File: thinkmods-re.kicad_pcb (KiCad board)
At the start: 2 copper layers, 30.5 x 68.1 mm, 12 parts, among them J1 ExpressCard, J2 Bus_M.2_Socket_M, J3 Micro_SD_Card, U1 GL823K-HCY04

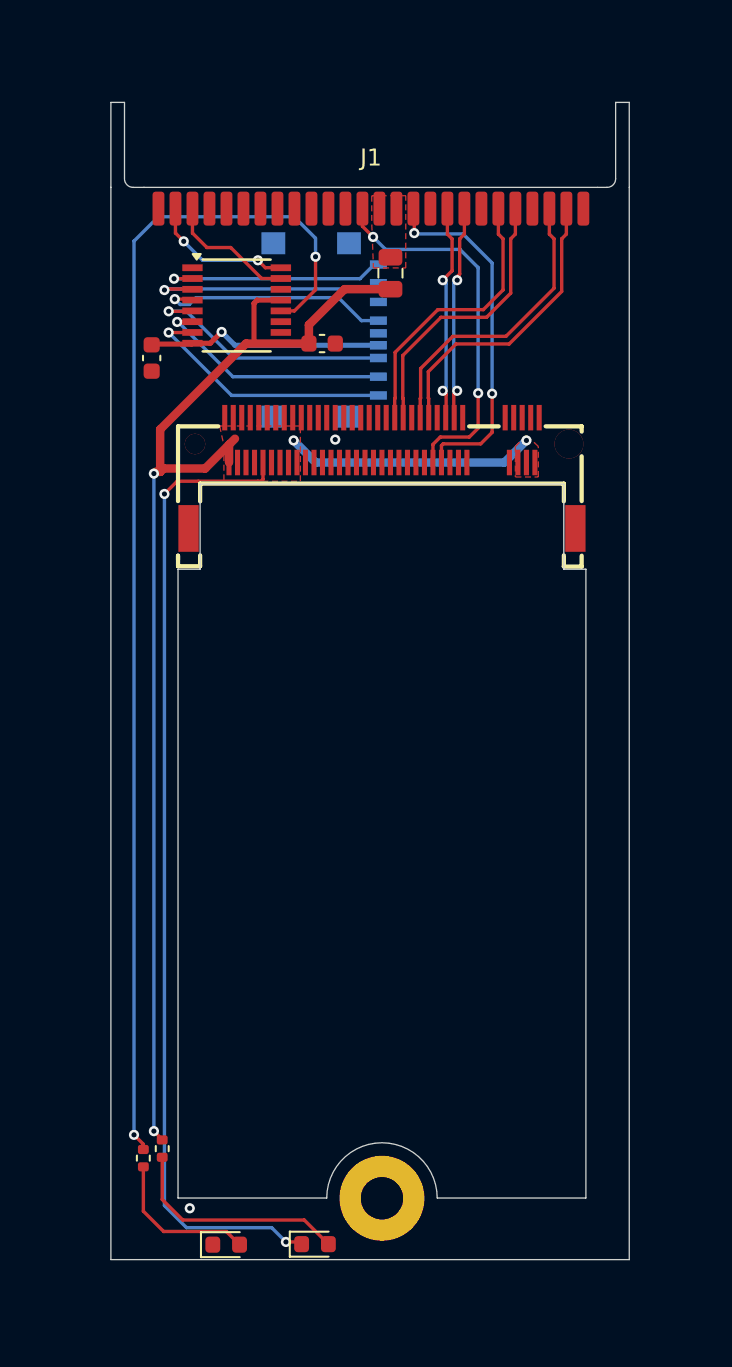
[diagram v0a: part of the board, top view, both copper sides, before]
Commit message: Add files via upload
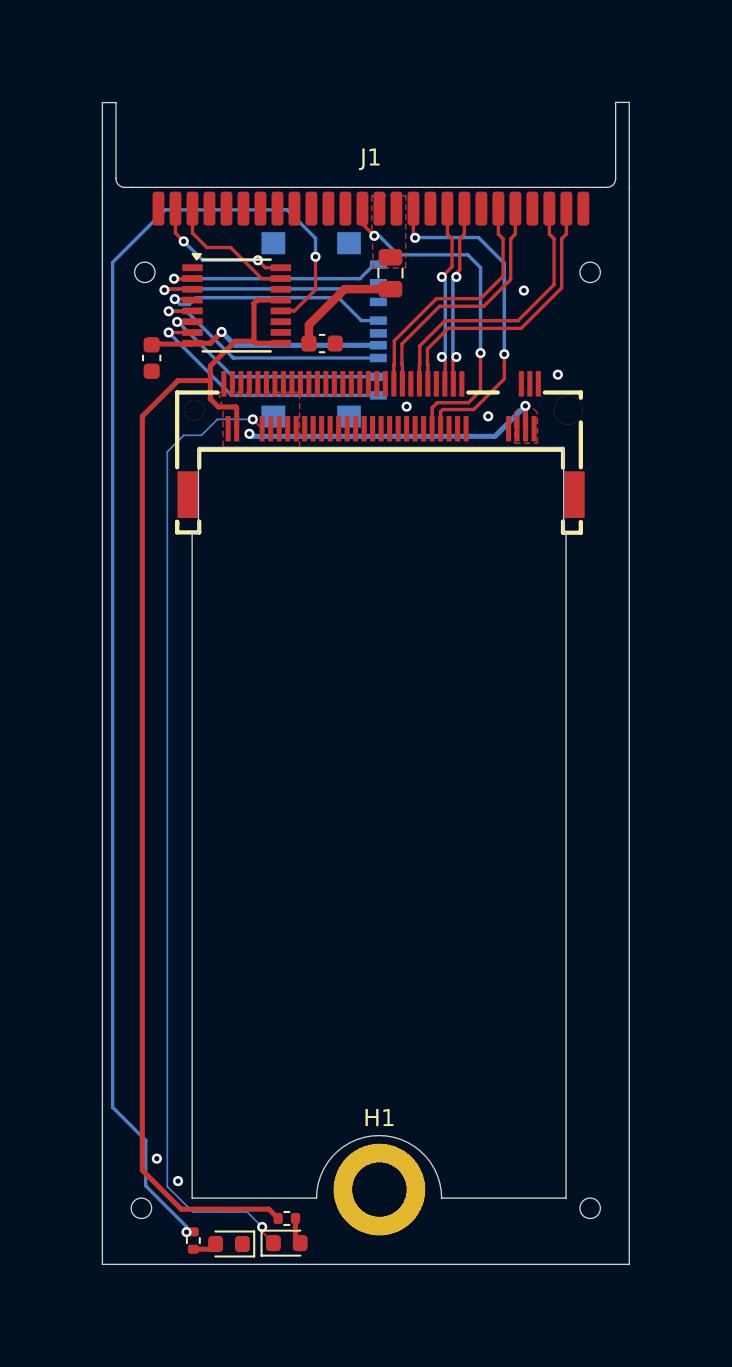
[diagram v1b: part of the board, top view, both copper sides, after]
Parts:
- removed the REF** at (169.8, 142.4)
- added H1: MountingHole_Pad_MP, Library:MountingHole_3.2mm_M3_Pad_small, F.Cu at (169.6, 141.9)
- added REF**: MountingHole_2.1mm, MountingHole:MountingHole_2.1mm, F.Cu at (182.0, 143.0)
- added REF**: MountingHole_2.1mm, MountingHole:MountingHole_2.1mm, F.Cu at (155.6, 143.0)
- added REF**: MountingHole_2.1mm, MountingHole:MountingHole_2.1mm, F.Cu at (155.8, 88.0)
- added REF**: MountingHole_2.1mm, MountingHole:MountingHole_2.1mm, F.Cu at (182.0, 88.0)
- moved R3 8.40 mm to (164.2, 143.6), turned to 180 degrees
- moved R4 5.67 mm to (158.7, 144.9)
- moved J2 1.99 mm to (169.7, 97.8)
- moved D2 1.66 mm to (164.2, 145.1)
- moved D1 0.17 mm to (160.8, 145.1), turned to 180 degrees
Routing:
- net Net-(D2-A): track 13.3 -> 1.56 mm
- net +3V3: track 86.5 -> 97.2 mm, vias 4 -> 2
- net /SD_LED: track 71.1 -> 78.8 mm
- net Net-(D1-A): track 9.09 -> 1.44 mm
- net /PCIe_RX+: track 16.6 -> 14.6 mm
- net /PCIe_RX-: track 16.6 -> 14.6 mm
- net /RCLK+: track 12.7 -> 10.8 mm
- net /RCLK-: track 12.9 -> 10.9 mm
- net /PERST: track 22.5 -> 20.7 mm
- net /PCIe_TX+: track 17.5 -> 16.2 mm
- net /PCIe_TX-: track 17.5 -> 16.2 mm
- net /CLKREQ: track 21.0 -> 20.0 mm
- net GND: vias 2 -> 6
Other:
- board size 30.5 x 68.1 mm -> 31 x 68.4 mm

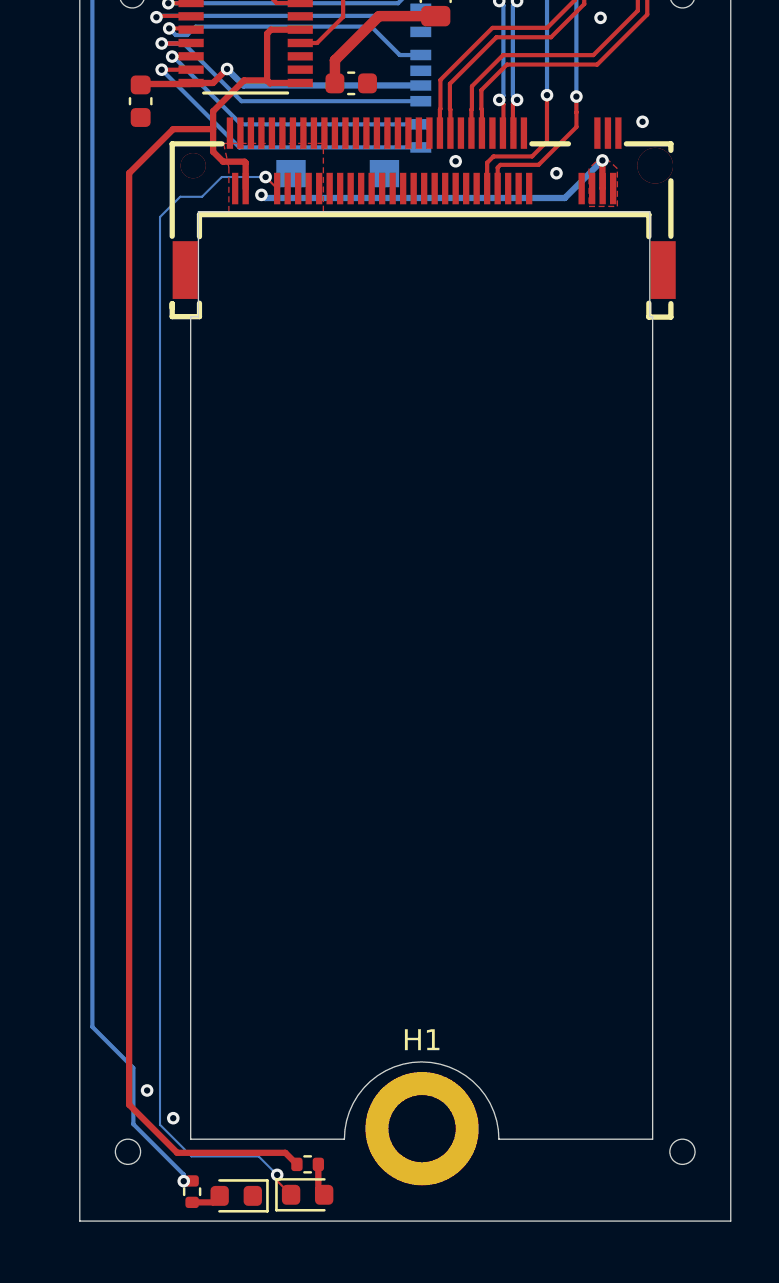
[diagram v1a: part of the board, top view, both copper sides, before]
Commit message: Add files via upload
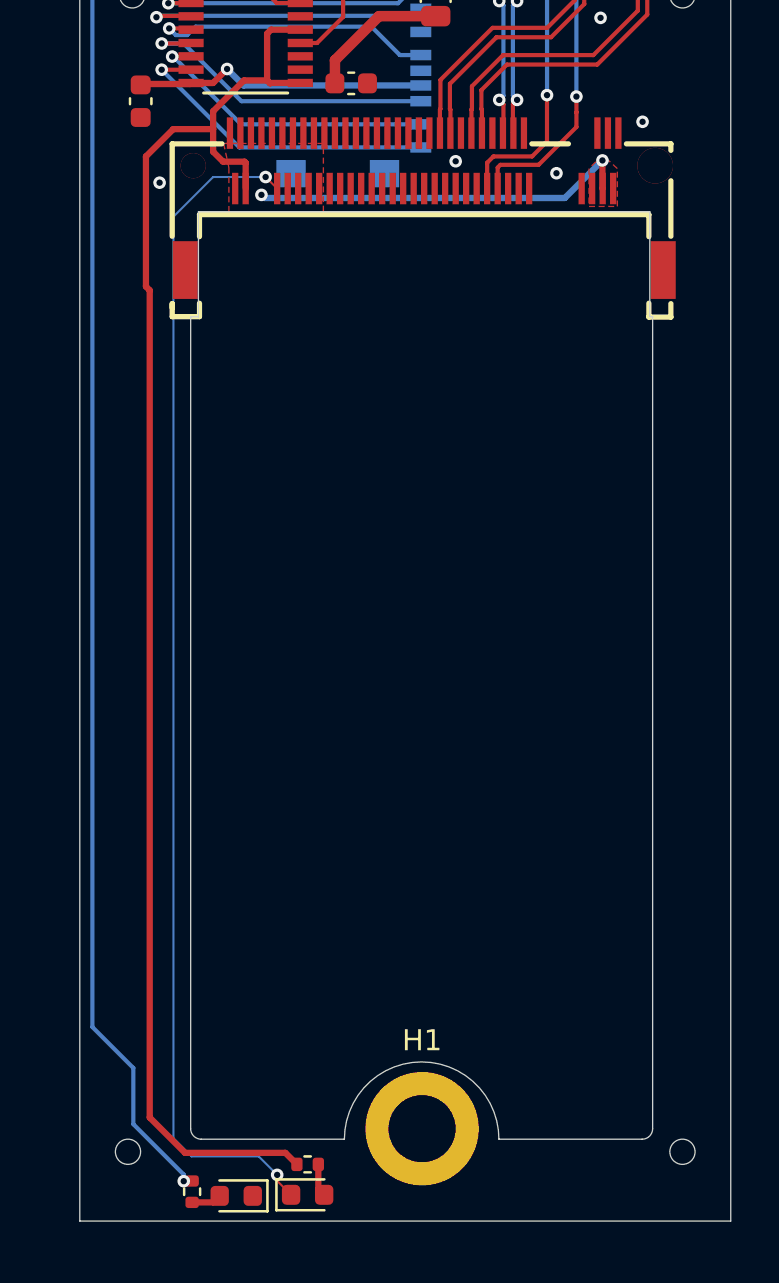
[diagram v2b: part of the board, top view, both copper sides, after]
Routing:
- net /PCIe_LED: track 57.6 -> 56.7 mm
- net +3V3: track 97.2 -> 96.3 mm
- net GND: vias 6 -> 5
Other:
- outline, holes or cut-outs redrawn
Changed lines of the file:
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@@
 		(pad_to_mask_clearance 0)
 		(allow_soldermask_bridges_in_footprints no)
-		(grid_origin 184.3 146.34)
+		(grid_origin 180.58 142.44)
 		(pcbplotparams
 			(layerselection 0x00010fc_ffffffff)
@@
 	)
 	(gr_arc
+		(start 159.079999 142.440001)
+		(mid 158.726446 142.293554)
+		(end 158.579999 141.940001)
+		(stroke
+			(width 0.05)
+			(type default)
+		)
+		(layer "Edge.Cuts")
+	)
+	(gr_arc
+		(start 180.58 141.94)
+		(mid 180.433553 142.293553)
+		(end 180.08 142.44)
+		(stroke
+			(width 0.05)
+			(type default)
+		)
+		(layer "Edge.Cuts")
+	)
+	(gr_arc
 		(start 165.9 142.44)
 		(mid 169.58 138.76)
@@
 	)
 	(gr_line
-		(start 180.58 142.44)
+		(start 180.58 141.94)
 		(end 180.58 103.27)
 		(stroke
@@
 	)
 	(gr_line
-		(start 158.58 142.44)
-		(end 165.9 142.44)
+		(start 159.079999 142.440001)
+		(end 165.899999 142.440001)
 		(stroke
 			(width 0.05)
@@
 	(gr_line
 		(start 173.26 142.44)
-		(end 180.58 142.44)
+		(end 180.08 142.44)
 		(stroke
 			(width 0.05)
@@
 	)
 	(gr_line
-		(start 158.58 142.44)
+		(start 158.58 141.94)
 		(end 158.58 103.28)
 		(stroke
@@
 	)
 	(via
-		(at 157.75 141.44)
+		(at 157.1 96.89)
 		(size 0.6)
 		(drill 0.3)
@@
 	)
 	(via
-		(at 156.505 140.12)
-		(size 0.6)
-		(drill 0.3)
-		(layers "F.Cu" "B.Cu")
-		(free yes)
-		(net 1)
-	)
-	(via
 		(at 176 96.44)
 		(size 0.6)
@@
 	)
 	(segment
-		(start 155.65 96.44)
-		(end 155.65 140.8)
+		(start 163.090001 143.09)
+		(end 163.640001 143.64)
 		(width 0.3)
 		(layer "F.Cu")
@@
 	)
 	(segment
+		(start 157.75 94.34)
+		(end 156.45 95.64)
+		(width 0.3)
+		(layer "F.Cu")
+		(net 3)
+	)
+	(segment
 		(start 161.12 92.02)
 		(end 162.22 92.02)
@@
 	)
 	(segment
+		(start 156.63 141.409239)
+		(end 158.310761 143.09)
+		(width 0.3)
+		(layer "F.Cu")
+		(net 3)
+	)
+	(segment
 		(start 159.65 94.34)
 		(end 159.65 93.49)
@@
 	)
 	(segment
+		(start 158.310761 143.09)
+		(end 163.090001 143.09)
+		(width 0.3)
+		(layer "F.Cu")
+		(net 3)
+	)
+	(segment
+		(start 156.45 101.835)
+		(end 156.63 102.015)
+		(width 0.3)
+		(layer "F.Cu")
+		(net 3)
+	)
+	(segment
 		(start 170.25 88.96)
 		(end 167.55 88.96)
@@
 	)
 	(segment
+		(start 156.45 95.64)
+		(end 156.45 101.835)
+		(width 0.3)
+		(layer "F.Cu")
+		(net 3)
+	)
+	(segment
 		(start 178.19 97.16)
 		(end 178.2 97.17)
@@
 	)
 	(segment
-		(start 163.090001 143.09)
-		(end 163.640001 143.64)
-		(width 0.3)
-		(layer "F.Cu")
-		(net 3)
-	)
-	(segment
-		(start 157.75 94.34)
-		(end 155.65 96.44)
-		(width 0.3)
-		(layer "F.Cu")
-		(net 3)
-	)
-	(segment
-		(start 157.94 143.09)
-		(end 163.090001 143.09)
+		(start 159.65 95.415)
+		(end 159.65 94.34)
 		(width 0.3)
 		(layer "F.Cu")
@@
 	)
 	(segment
-		(start 155.65 140.8)
-		(end 157.94 143.09)
-		(width 0.3)
-		(layer "F.Cu")
-		(net 3)
-	)
-	(segment
-		(start 159.65 95.415)
-		(end 159.65 94.34)
+		(start 156.63 102.015)
+		(end 156.63 141.409239)
 		(width 0.3)
 		(layer "F.Cu")
@@
 	)
 	(segment
-		(start 160.065 96.62)
-		(end 162.15 96.62)
-		(width 0.1)
-		(layer "B.Cu")
-		(net 5)
-	)
-	(segment
-		(start 159.125 97.56)
-		(end 160.065 96.62)
-		(width 0.1)
-		(layer "B.Cu")
-		(net 5)
-	)
-	(segment
-		(start 161.82 143.26)
-		(end 158.622183 143.26)
+		(start 158.622183 143.26)
+		(end 157.76 142.397817)
 		(width 0.1)
 		(layer "B.Cu")
@@
 	)
 	(segment
-		(start 158.622183 143.26)
-		(end 157.12 141.757817)
+		(start 157.76 98.51)
+		(end 159.65 96.62)
 		(width 0.1)
 		(layer "B.Cu")
@@
 	)
 	(segment
-		(start 157.12 98.525)
-		(end 158.085 97.56)
+		(start 162.7 144.14)
+		(end 161.82 143.26)
 		(width 0.1)
 		(layer "B.Cu")
@@
 	)
 	(segment
-		(start 157.12 141.757817)
-		(end 157.12 98.525)
+		(start 159.65 96.62)
+		(end 162.15 96.62)
 		(width 0.1)
 		(layer "B.Cu")
@@
 	)
 	(segment
-		(start 158.085 97.56)
-		(end 159.125 97.56)
+		(start 161.82 143.26)
+		(end 158.622183 143.26)
 		(width 0.1)
 		(layer "B.Cu")
@@
 	)
 	(segment
-		(start 162.7 144.14)
-		(end 161.82 143.26)
+		(start 157.76 142.397817)
+		(end 157.76 98.51)
 		(width 0.1)
 		(layer "B.Cu")
